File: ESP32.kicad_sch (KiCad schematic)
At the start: 36 parts, among them J1 Conn_01x06, J3 USB_C_Receptacle_USB2.0_16P, J4 Conn_01x03, J5 Jack-DC, Q3 SS8050, Q4 SS8050, U1 TLV75733PDBV, U2 ESP32-WROOM-32E, U3 CP2102N-A02-GQFN24

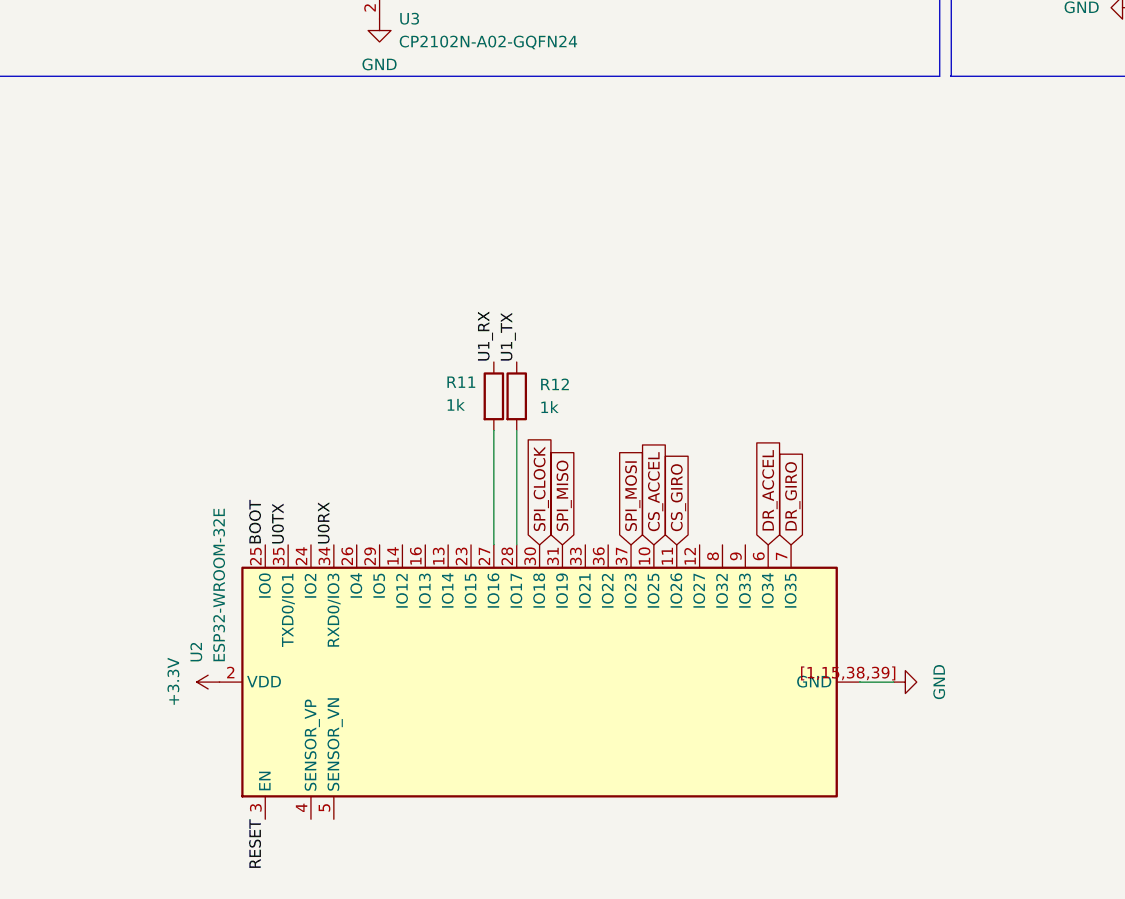
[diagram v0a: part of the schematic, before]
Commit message: Esquematico preparado para revision
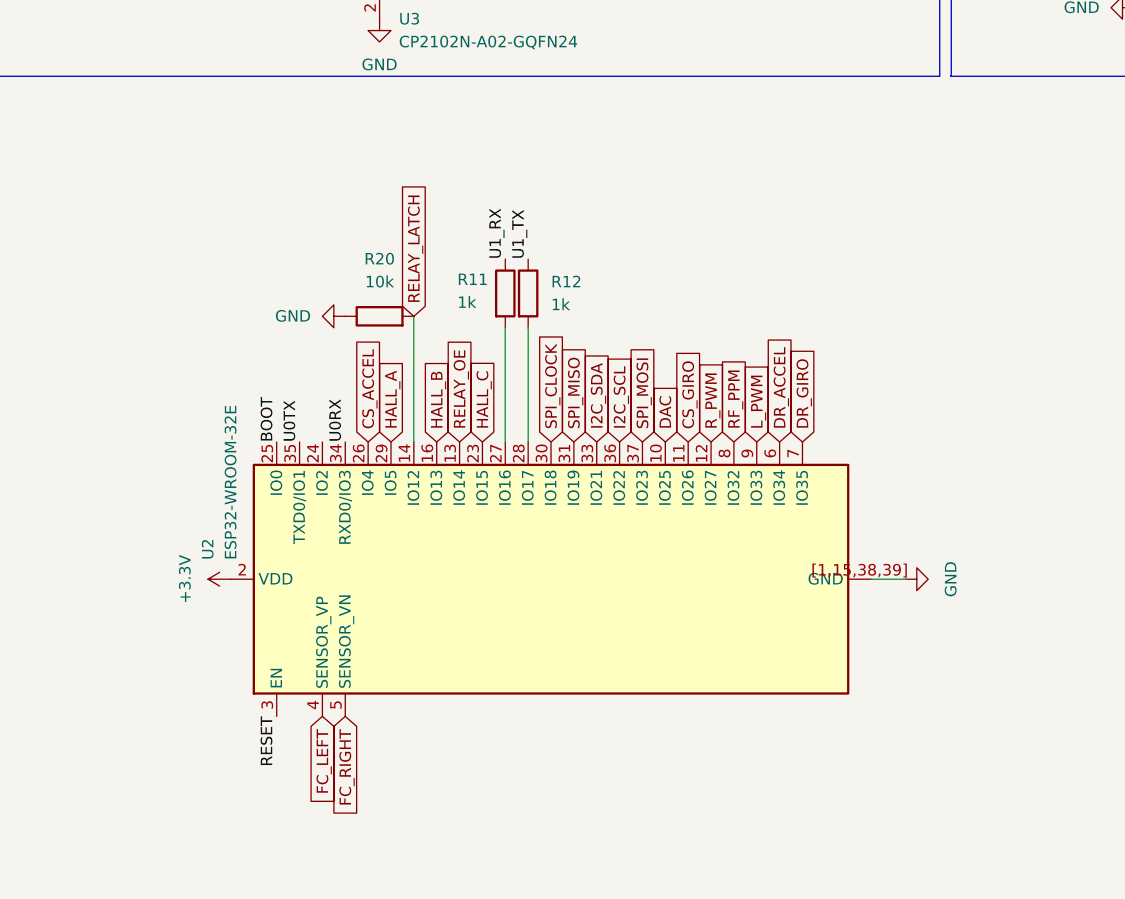
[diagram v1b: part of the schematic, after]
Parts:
- added R20: 10k, symbol Device:R
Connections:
- net CS_ACCEL: now also U2.26 (IO4); no longer U2.10 (IO25)
- net GND: now also R20.1
- net R_PWM: now reaches U2.12 (IO27)
- net RELAY_OE: now reaches U2.13 (IO14)
- net RELAY_LATCH: now reaches U2.14 (IO12)
- net RELAY_LATCH: now also R20.2
- net HALL_B: now reaches U2.16 (IO13)
- net HALL_C: now reaches U2.23 (IO15)
- net HALL_A: now reaches U2.29 (IO5)
- net I2C_SDA: now reaches U2.33 (IO21)
- net I2C_SCL: now reaches U2.36 (IO22)
- net FC_LEFT: now reaches U2.4 (SENSOR_VP)
- net FC_RIGHT: now reaches U2.5 (SENSOR_VN)
- net RF_PPM: now reaches U2.8 (IO32)
- net L_PWM: now reaches U2.9 (IO33)
- new net DAC: U2.10 (IO25)
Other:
- moved on the sheet: R11, R12, U2
